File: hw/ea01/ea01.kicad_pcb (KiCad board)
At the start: 2 copper layers, 100 x 45 mm, 195 parts, among them J1 Screw_Terminal_01x02, J10 Screw_Terminal_01x02, J11 Screw_Terminal_01x02, J12 Screw_Terminal_01x03, J13 Conn_01x02_Pin, J14 Conn_01x02_Pin, J15 Conn_01x02_Pin, J16 Conn_01x02_Pin, J17 Conn_01x02_Pin, J18 Conn_01x02_Pin, J19 Conn_01x02_Pin, J2 USB_B, J3 Conn_01x05_Pin, J4 Screw_Terminal_01x02, J5 Screw_Terminal_01x02, J6 Conn_01x02_Pin, J7 Conn_01x03_Pin, J8 Conn_01x03_Pin, J9 Conn_01x03_Pin, K1 G5NB, K2 G5NB, Q1 BC817, Q11 BC817, Q2 BC817, Q3 BC817, Q4 BC817, Q5 BC817, Q6 BC817, Q7 BC817, Q9 BC817, SW1 SW_Push, SW2 SW_Push, SW3 SW_Push, SW4 SW_Push, U1 RP2040, U11 W25Q32JVSS, U12 SN75176AP, U13 PC817, U14 PC817, U2 PCF8563T, U3 NUP2202, U4 MC34063AD, U6 AMS1117-3.3, U8 CAT24C256, U9 74HC14, Y1 12Mhz, Y3 32.768Khz

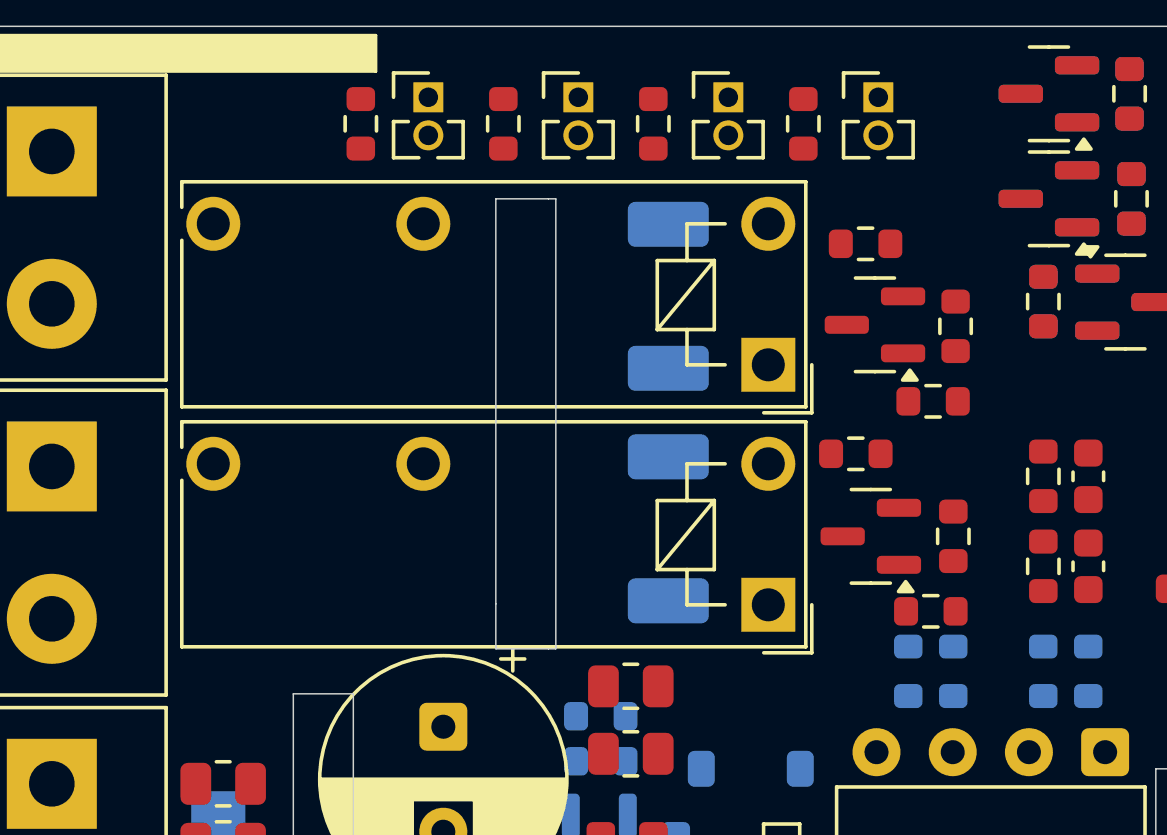
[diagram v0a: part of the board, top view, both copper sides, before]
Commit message: update..
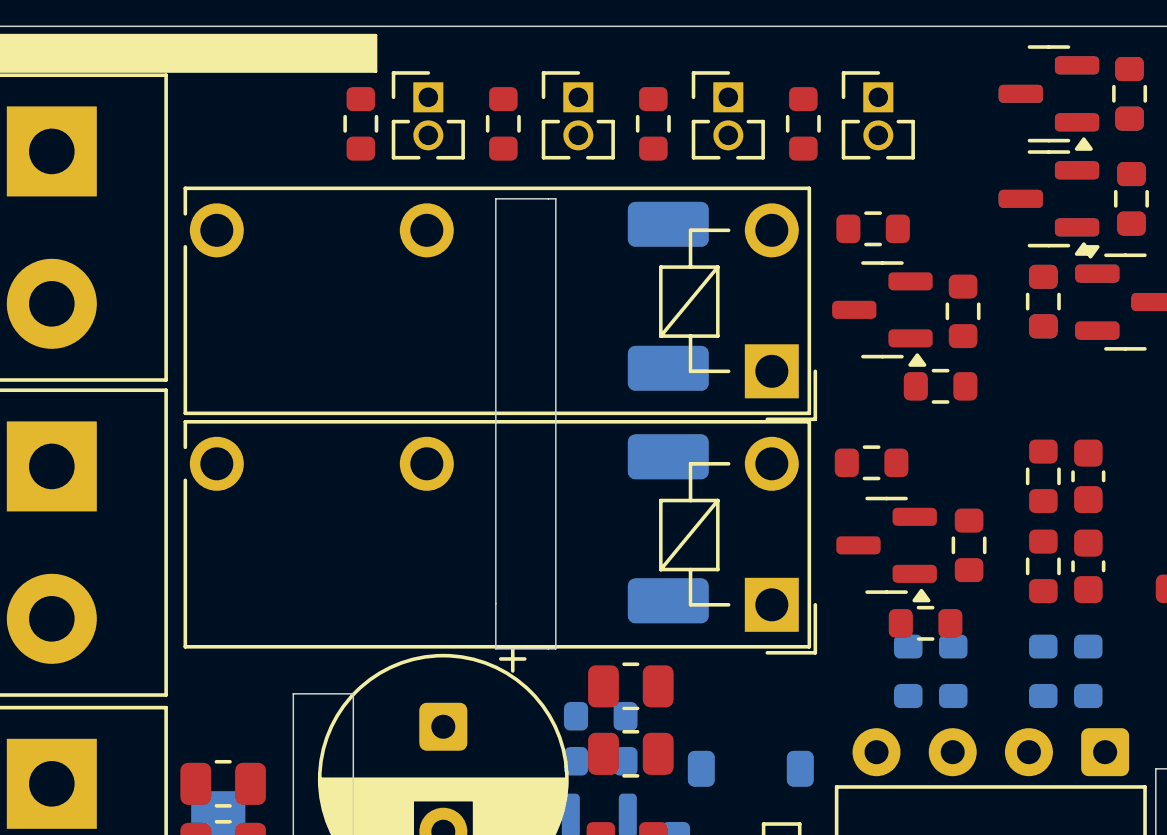
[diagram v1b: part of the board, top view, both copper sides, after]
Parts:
- moved Q11 0.60 mm to (97.5, 66.3)
- moved R79 0.60 mm to (100.3, 66.3)
- moved R80 0.60 mm to (97.0, 63.5)
- moved Q9 0.56 mm to (97.4, 58.5)
- moved R69 0.56 mm to (99.3, 61.0)
- moved R70 0.56 mm to (100.1, 58.5)
- moved R71 0.56 mm to (97.1, 55.8)
- moved R78 0.44 mm to (98.8, 68.9)
- moved K1 0.25 mm to (93.7, 60.5)
- moved K2 0.12 mm to (93.7, 68.3)
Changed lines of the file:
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@@
 	(footprint "Package_TO_SOT_SMD:SOT-23"
 		(layer "F.Cu")
-		(at 97 66 180)
+		(at 97.525 66.3 180)
 		(descr "SOT, 3 Pin (JEDEC TO-236 Var AB https://www.jedec.org/document_search?search_api_views_fulltext=TO-236), generated with kicad-footprint-generator ipc_gullwing_generator.py")
 		(tags "SOT TO_SOT_SMD")
@@
 	(footprint "Resistor_SMD:R_0603_1608Metric"
 		(layer "F.Cu")
-		(at 96.5 63.25)
+		(at 97.025 63.55)
 		(descr "Resistor SMD 0603 (1608 Metric), square (rectangular) end terminal, IPC-7351 nominal, (Body size source: IPC-SM-782 page 72, https://www.pcb-3d.com/wordpress/wp-content/uploads/ipc-sm-782a_amendment_1_and_2.pdf), generated with kicad-footprint-generator")
 		(tags "resistor")
@@
 	(footprint "Resistor_SMD:R_0603_1608Metric"
 		(layer "F.Cu")
-		(at 99 68.5 180)
+		(at 98.825 68.9 180)
 		(descr "Resistor SMD 0603 (1608 Metric), square (rectangular) end terminal, IPC-7351 nominal, (Body size source: IPC-SM-782 page 72, https://www.pcb-3d.com/wordpress/wp-content/uploads/ipc-sm-782a_amendment_1_and_2.pdf), generated with kicad-footprint-generator")
 		(tags "resistor")
@@
 	(footprint "Relay_THT:Relay_SPST_Omron_G5NB"
 		(layer "F.Cu")
-		(at 93.5825 60.2825 180)
+		(at 93.7 60.5 180)
 		(descr "PCB Power Relay, SPST-NO, 7A (250 VAC), 5A (30 VDC), 20.5x7.2x15.3mm max")
 		(tags "Omron G5NB Relay SPST-NO")
@@
 	(footprint "Resistor_SMD:R_0603_1608Metric"
 		(layer "F.Cu")
-		(at 96.825 56.25)
+		(at 97.075 55.75)
 		(descr "Resistor SMD 0603 (1608 Metric), square (rectangular) end terminal, IPC-7351 nominal, (Body size source: IPC-SM-782 page 72, https://www.pcb-3d.com/wordpress/wp-content/uploads/ipc-sm-782a_amendment_1_and_2.pdf), generated with kicad-footprint-generator")
 		(tags "resistor")
@@
 	(footprint "Resistor_SMD:R_0603_1608Metric"
 		(layer "F.Cu")
-		(at 99.825 59 90)
+		(at 100.075 58.5 90)
 		(descr "Resistor SMD 0603 (1608 Metric), square (rectangular) end terminal, IPC-7351 nominal, (Body size source: IPC-SM-782 page 72, https://www.pcb-3d.com/wordpress/wp-content/uploads/ipc-sm-782a_amendment_1_and_2.pdf), generated with kicad-footprint-generator")
 		(tags "resistor")
@@
 	(footprint "Relay_THT:Relay_SPST_Omron_G5NB"
 		(layer "F.Cu")
-		(at 93.5825 68.2825 180)
+		(at 93.7 68.2825 180)
 		(descr "PCB Power Relay, SPST-NO, 7A (250 VAC), 5A (30 VDC), 20.5x7.2x15.3mm max")
 		(tags "Omron G5NB Relay SPST-NO")
@@
 	(footprint "Resistor_SMD:R_0603_1608Metric"
 		(layer "F.Cu")
-		(at 99.75 66 90)
+		(at 100.275 66.3 90)
 		(descr "Resistor SMD 0603 (1608 Metric), square (rectangular) end terminal, IPC-7351 nominal, (Body size source: IPC-SM-782 page 72, https://www.pcb-3d.com/wordpress/wp-content/uploads/ipc-sm-782a_amendment_1_and_2.pdf), generated with kicad-footprint-generator")
 		(tags "resistor")
@@
 	(footprint "Resistor_SMD:R_0603_1608Metric"
 		(layer "F.Cu")
-		(at 99.075 61.5 180)
+		(at 99.325 61 180)
 		(descr "Resistor SMD 0603 (1608 Metric), square (rectangular) end terminal, IPC-7351 nominal, (Body size source: IPC-SM-782 page 72, https://www.pcb-3d.com/wordpress/wp-content/uploads/ipc-sm-782a_amendment_1_and_2.pdf), generated with kicad-footprint-generator")
 		(tags "resistor")
@@
 	(footprint "Package_TO_SOT_SMD:SOT-23"
 		(layer "F.Cu")
-		(at 97.1375 58.95 180)
+		(at 97.3875 58.45 180)
 		(descr "SOT, 3 Pin (JEDEC TO-236 Var AB https://www.jedec.org/document_search?search_api_views_fulltext=TO-236), generated with kicad-footprint-generator ipc_gullwing_generator.py")
 		(tags "SOT TO_SOT_SMD")
